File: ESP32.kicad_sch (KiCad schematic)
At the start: 40 parts, among them J2 Conn_01x04_Socket, U2 ESP32-C3FH4, U4 TS-1187A-B-A-B, U5 TS-1187A-B-A-B, U58 TS-1187A-B-A-B, U59 YTC-TC16-30, U60 AMS1117-3_3, U73 TS-1187A-B-A-B, X1 CF4040M00015001

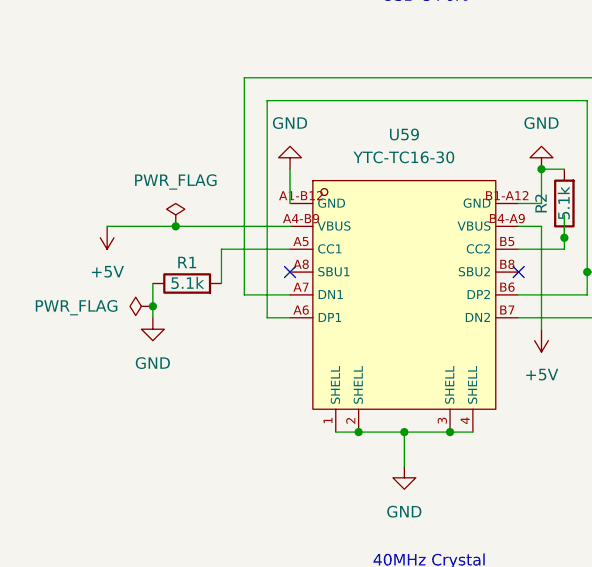
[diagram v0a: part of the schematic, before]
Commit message: fixed routing
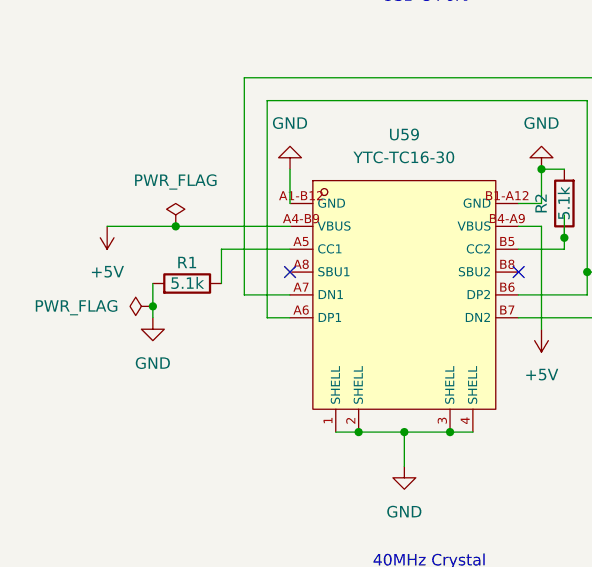
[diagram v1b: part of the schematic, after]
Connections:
- net GND: now also R1.2; no longer R1.1
- net at U59.A5 (CC1): now also R1.1; no longer R1.2
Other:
- moved on the sheet: R1
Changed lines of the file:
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@@
 	(symbol
 		(lib_id "Device:R")
-		(at 27.94 52.07 90)
+		(at 27.94 52.07 270)
+		(mirror x)
 		(unit 1)
 		(exclude_from_sim no)
